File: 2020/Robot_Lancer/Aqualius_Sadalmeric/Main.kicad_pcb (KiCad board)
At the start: 2 copper layers, 100 x 100 mm, 323 parts, among them J1 SERIAL0, J10 I/O_Vdd, J11 ENC0, J12 ENC1, J13 ENC2, J14 ENC3, J15 5Vin, J16 EMERGENCY, J17 MOTOR0, J18 MOTOR1, J19 MOTOR2, J2 ADC, J20 MOTOR3, J21 MOTOR4, J22 MOTOR5, J23 BATT_IN, J24 BATT_IN, J25 FUSE, J3 SWD, J4 CAN, J5 ADC_Vdd, J6 SERIAL1, J7 CAN, J8 VALVE, J9 SERIAL2, Q1 NPN, Q10 NVMFD5C446NLT1G, Q11 FET_N, Q12 NVMFD5C446NLT1G, Q13 NVMFD5C446NLT1G, Q14 NVMFD5C446NLT1G, Q15 NVMFD5C446NLT1G, Q16 NVMFD5C446NLT1G, Q17 NVMFD5C446NLT1G, Q18 FET_P, Q3 FET_P, Q4 FET_P, Q5 NVMFD5C446NLT1G, Q6 NVMFD5C446NLT1G, Q7 NVMFD5C446NLT1G, Q8 NVMFD5C446NLT1G, Q9 NVMFD5C446NLT1G, SW1 RESET, SW10 TOGGLESW1, SW11 TOGGLESW2, SW12 TOGGLESW3, SW2 TOGGLESW0, SW3 SW0, SW4 SW1, SW5 Control-Power_SW, SW6 SW2, SW7 SW3, SW8 EMERGENCY_SW, SW9 MAIN_SW, U1 MAX3051, U10 BD9G101G, U11 CCG30-24-12, U12 NCP5104, U13 NCP5104, U14 NCP5104, U15 NCP5104, U16 NCP5104, U17 NCP5104, U18 V23086-C1001, U19 NCP5104, U2 AP3211, U20 NCP5104, U21 NCP5104, U22 NCP5104, U23 NCP5104, U24 NCP5104, U25 LOGO, U26 7805, U27 TBD62083A, U3 MCP2221A, U4 AQM0802, U5 AZ1086H, U6 STM32F407VG, U7 OSTBABS4C2B, U8 ADRESS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

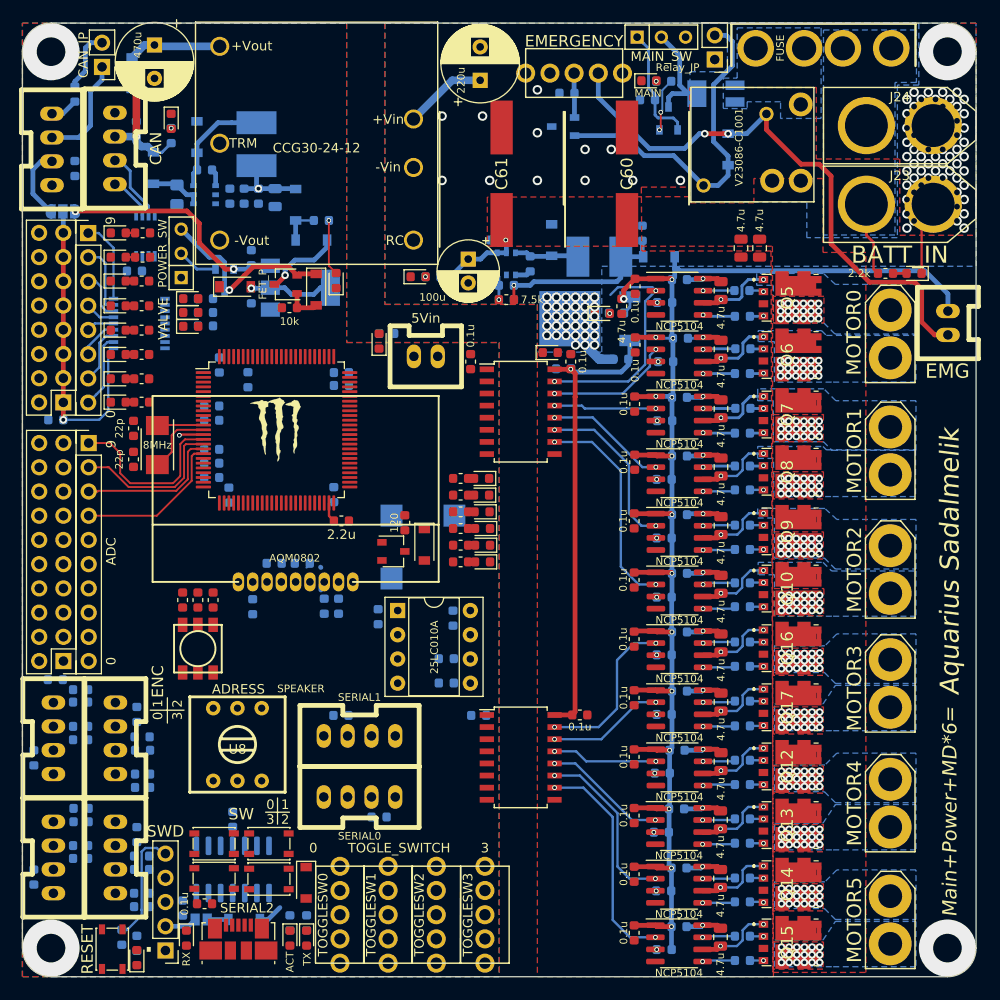
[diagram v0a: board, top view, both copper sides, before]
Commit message: アロエ
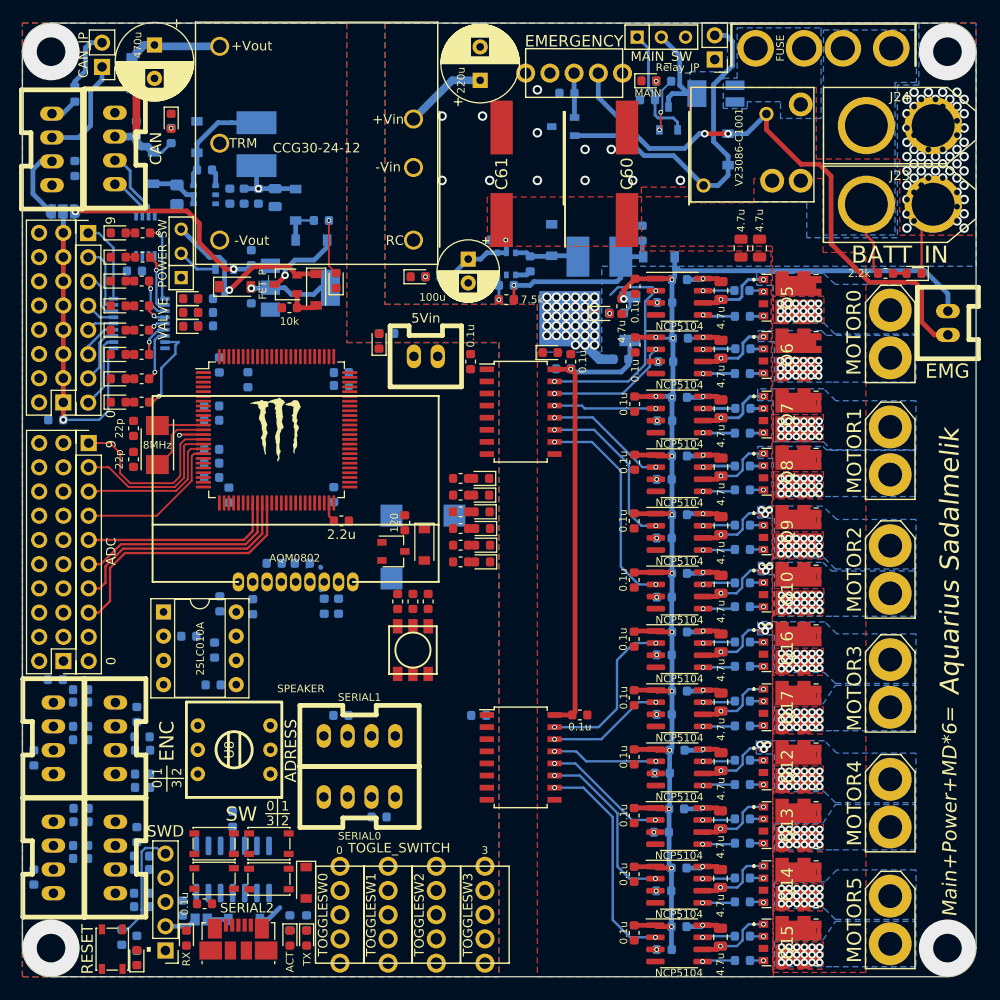
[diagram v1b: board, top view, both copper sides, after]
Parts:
- moved U9 24.6 mm to (50.8, 99.8)
- moved C40 24.5 mm to (56.7, 98.9), turned to 90 degrees
- moved R56 24.5 mm to (56.0, 107.4)
- moved R55 24.3 mm to (56.1, 103.8), turned to 270 degrees
- moved R37 22.6 mm to (77.0, 98.7)
- moved U7 22.6 mm to (77.0, 103.8)
- moved R36 22.6 mm to (78.5, 98.7)
- moved R38 22.6 mm to (75.3, 98.7)
- moved R54 20.0 mm to (53.5, 102.3), turned to 0 degrees
- moved U8 0.65 mm to (58.2, 114.2), turned to 270 degrees
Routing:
- net /PB1_ADC12_IN9: track 0.00 -> 27.5 mm
- net /PB0_ADC12_IN8: track 0.00 -> 24.8 mm
- net /PC5_ADC12_IN15: track 0.00 -> 22.2 mm
- net /PC4_ADC12_IN14: track 0.00 -> 20.5 mm
- net /PA12_IO: track 0.00 -> 9.26 mm, vias 0 -> 1
- net /PE0_IO: track 0.00 -> 8.05 mm, vias 0 -> 1
- net /PE1_IO: track 0.00 -> 6.09 mm, vias 0 -> 1
- net /PA11_IO: track 0.00 -> 5.58 mm, vias 0 -> 1
- net /PE12_IO: track 0.00 -> 4.28 mm, vias 0 -> 1
- net /PA8_IO: track 0.00 -> 3.67 mm, vias 0 -> 1
- net /PE15_IO: track 0.00 -> 2.47 mm, vias 0 -> 1
- net /PA4_IO: track 0.00 -> 1.95 mm, vias 0 -> 1
- net Net-(D22-Pad2): track 0.00 -> 0.88 mm
- net Net-(D21-Pad2): track 0.00 -> 0.88 mm
- net Net-(D13-Pad2): track 0.00 -> 0.88 mm
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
